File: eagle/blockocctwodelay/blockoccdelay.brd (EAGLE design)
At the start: 91.4 x 93.7 mm, 58 parts, among them IC1 74LS14N, IC2 555, IC3 555, IC4 555, IC5 555, IC6 555, IC7 555, X1 MKDSN1,5/2-5,08, X10 MKDSN1,5/2-5,08, X11 MKDSN1,5/2-5,08, X12 MKDSN1,5/2-5,08, X13 MKDSN1,5/2-5,08, X14 MKDSN1,5/2-5,08, X2 MKDSN1,5/2-5,08, X3 MKDSN1,5/2-5,08, X4 MKDSN1,5/2-5,08, X5 MKDSN1,5/2-5,08, X6 MKDSN1,5/2-5,08, X7 MKDSN1,5/2-5,08, X8 MKDSN1,5/2-5,08, X9 MKDSN1,5/2-5,08

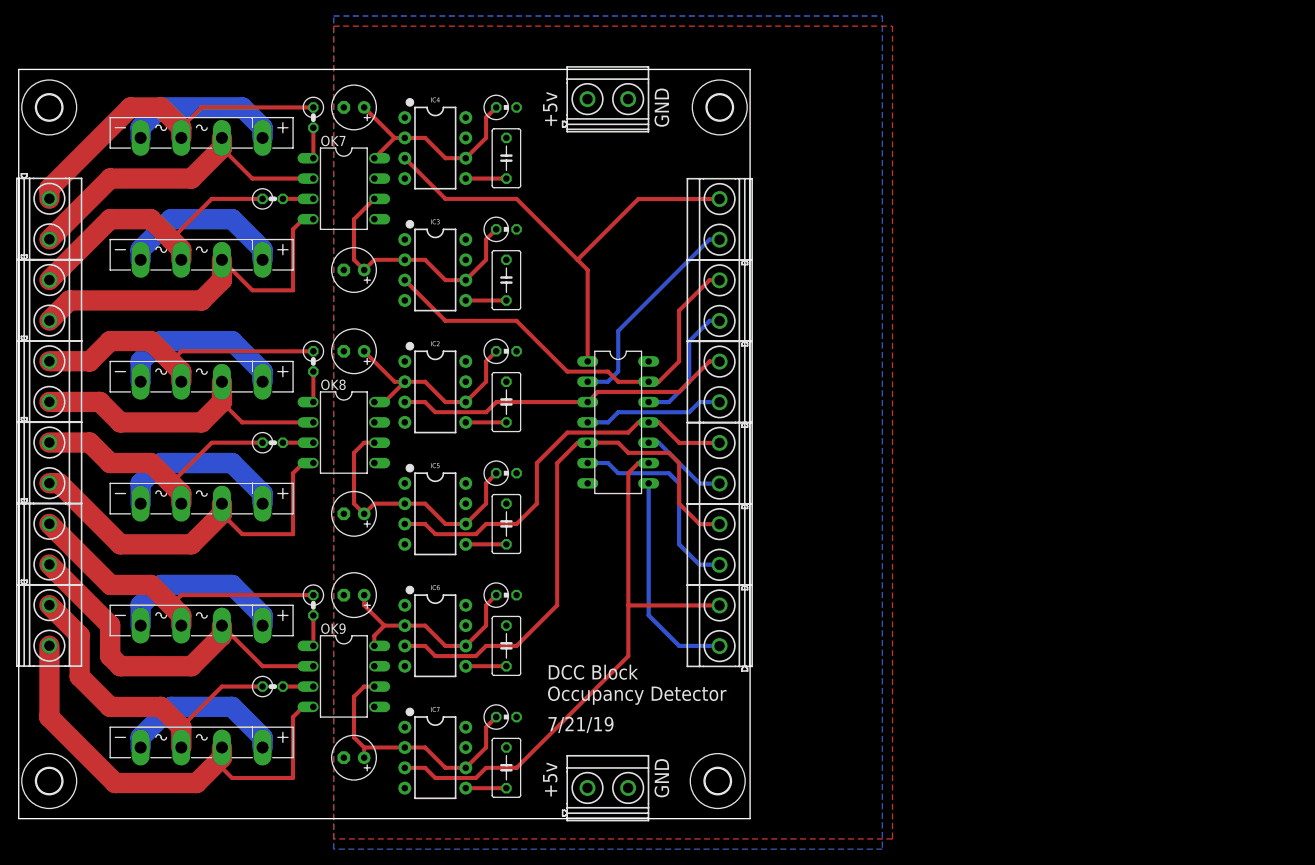
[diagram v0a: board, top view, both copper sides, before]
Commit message: periodic checkin
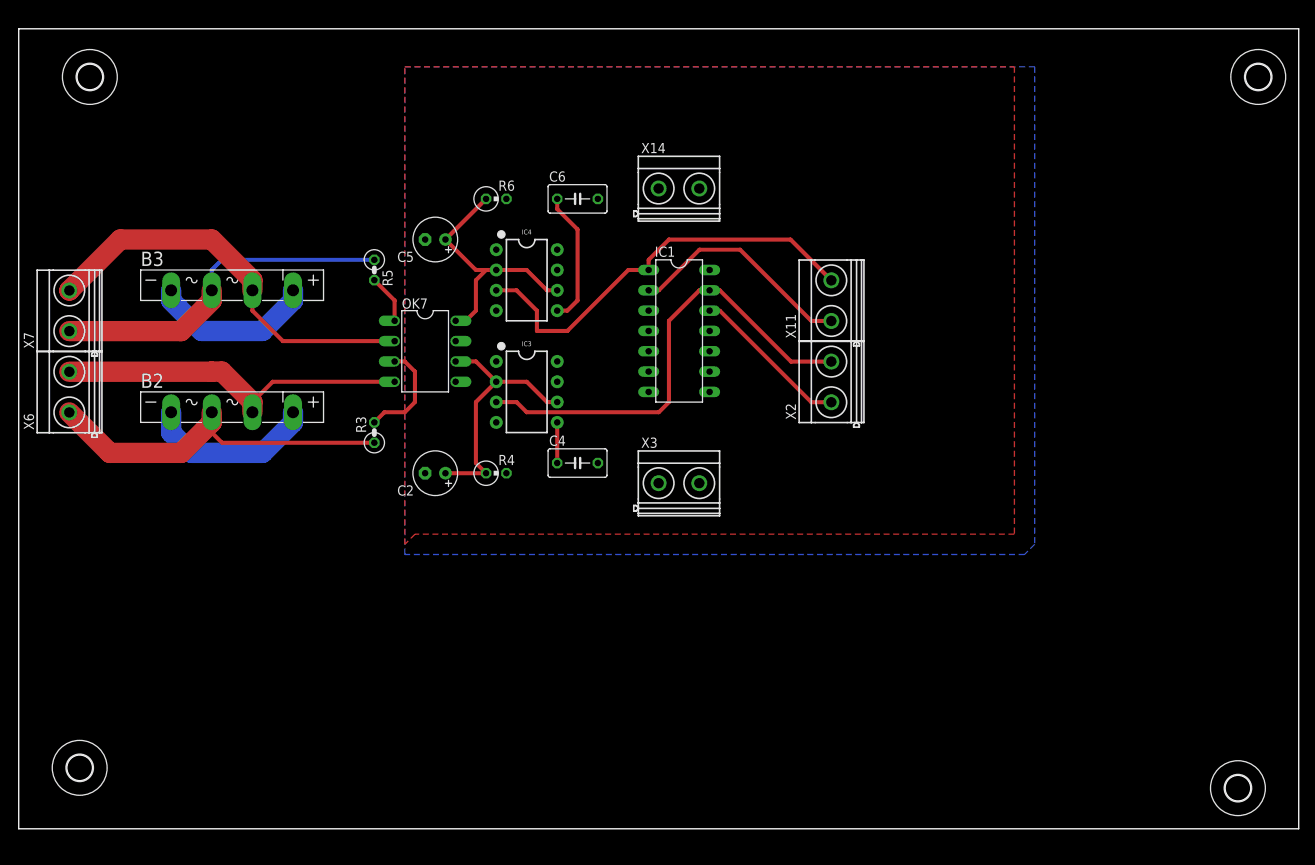
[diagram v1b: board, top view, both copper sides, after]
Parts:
- removed B1, B4, B5, B6: (no value), rectifier:GBU4S
- removed C1, C11, C7, C9: 10uf, resistor:E2,5-6
- removed C10, C12, C3, C8: 0.01uf, resistor:C050-035X075
- removed IC2, IC5, IC6, IC7: 555, SparkFun-IC-Special-Function:DIP08
- removed OK8, OK9: LTV826, optocoupler:DIL08
- removed R1, R11, R7, R9: 33r, resistor:0207/2V
- removed R10, R12, R2, R8: 120k, resistor:0309V
- removed X1, X10, X12, X13, X4, X5, X8, X9: MKDSN1,5/2-5,08, con-phoenix-508:MKDSN1,5/2-5,08
- moved H4 171.2 mm to (152.4, 5.08)
- moved H2 117.9 mm to (8.89, 94.0)
- moved H3 67.4 mm to (154.9, 94.0)
- moved X3 39.1 mm to (82.5, 43.2)
- moved R3 31.9 mm to (44.5, 49.5), turned to 90 degrees
- moved R4 30.5 mm to (59.7, 44.5)
- moved C2 27.4 mm to (52.1, 44.5)
- moved C4 24.5 mm to (69.8, 45.7), turned to 0 degrees
- moved OK7 22.7 mm to (50.8, 59.7)
- moved R5 20.5 mm to (44.5, 69.8)
- moved IC4 20.1 mm to (63.5, 68.6)
- moved B2 19.4 mm to (26.7, 52.1)
- moved B3 19.4 mm to (26.7, 67.3)
- moved C5 19.4 mm to (52.1, 73.7)
- moved IC3 19.0 mm to (63.5, 54.6)
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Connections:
- removed net DCC3: B1.AC2, R1.1, X1.1
- removed net DCC4: B4.AC2, R7.1, X8.1
- removed net DCC5: B5.AC2, R9.1, X9.1
- removed net DCC6: B6.AC2, R11.1, X10.1
- removed net N$1: B1.+, B1.-
- removed net N$16: B5.+, B5.-
- removed net N$17: OK9.1, R9.2
- removed net N$18: C10.1, IC6.5
- removed net N$19: B6.+, B6.-
- removed net N$2: OK8.1, R1.2
- removed net N$20: OK9.3, R11.2
- removed net N$21: C12.1, IC7.5
- removed net N$23: IC1.4, X12.1
- removed net N$24: IC1.6, X13.1
- removed net N$3: C3.1, IC2.5
- removed net N$5: B4.+, B4.-
- removed net N$6: OK8.3, R7.2
- removed net N$7: IC1.10, X4.1
- removed net N$8: C8.1, IC5.5
- removed net N$9: IC1.8, X5.1
- removed net RAW3: IC1.3, IC2.3, X12.2
- removed net RAW4: IC1.11, IC5.3, X4.2
- removed net RAW5: IC1.5, IC6.3, X13.2
- removed net RAW6: IC1.9, IC7.3, X5.2
- removed net TRI: C1.+, IC2.2, IC2.6, OK8.8, R2.1
- removed net TRI3: C7.+, IC5.2, IC5.6, OK8.6, R8.1
- removed net TRI4: C9.+, IC6.2, IC6.6, OK9.8, R10.1
- removed net TRI5: C11.+, IC7.2, IC7.6, OK9.6, R12.1
- removed net TRK3: B1.AC1, OK8.2, X1.2
- removed net TRK4: B4.AC1, OK8.4, X8.2
- removed net TRK5: B5.AC1, OK9.2, X9.2
- removed net TRK6: B6.AC1, OK9.4, X10.2
- net +5V: no longer IC2.4, IC2.8, IC5.4, IC5.8, IC6.4, IC6.8, IC7.4, IC7.8, R10.2, R12.2, R2.2, R8.2
- net GND: no longer C1.-, C10.2, C11.-, C12.2, C3.2, C7.-, C8.2, C9.-, IC2.1, IC5.1, IC6.1, IC7.1, OK8.5, OK8.7, OK9.5, OK9.7
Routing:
- net RAW6: track 72.1 -> 0.00 mm
- net RAW5: track 68.5 -> 0.00 mm
- net TRK6: track 57.9 -> 0.00 mm
- net RAW4: track 49.7 -> 0.00 mm
- net TRK4: track 48.2 -> 0.00 mm
- net TRK5: track 45.5 -> 0.00 mm
- net RAW3: track 42.5 -> 0.00 mm
- net DCC5: track 40.8 -> 0.00 mm
- net DCC6: track 40.6 -> 0.00 mm
- net TRK3: track 38.7 -> 0.00 mm
- net DCC3: track 38.7 -> 0.00 mm
- net DCC4: track 33.9 -> 0.00 mm
- net TRI3: track 33.4 -> 0.00 mm
- net TRI5: track 32.9 -> 0.00 mm
- net TRI: track 28.1 -> 0.00 mm
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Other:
- board size 91.4 x 93.7 mm -> 160 x 100 mm
- board text removed: "+5v"
- board text removed: "7/21/19"
- board text removed: "DCC Block Occupancy Detector"
- board text removed: "GND"
